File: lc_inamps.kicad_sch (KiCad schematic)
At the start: 30 parts, among them J14 Conn_01x04_Male, J15 Conn_01x04_Male, J16 Conn_01x04, J17 Conn_01x08, J18 Conn_01x04_Male, J19 Conn_01x04_Male, U3 MCP6N11R, U4 MCP6N11R, U5 MCP6N11R, U6 MCP6N11R

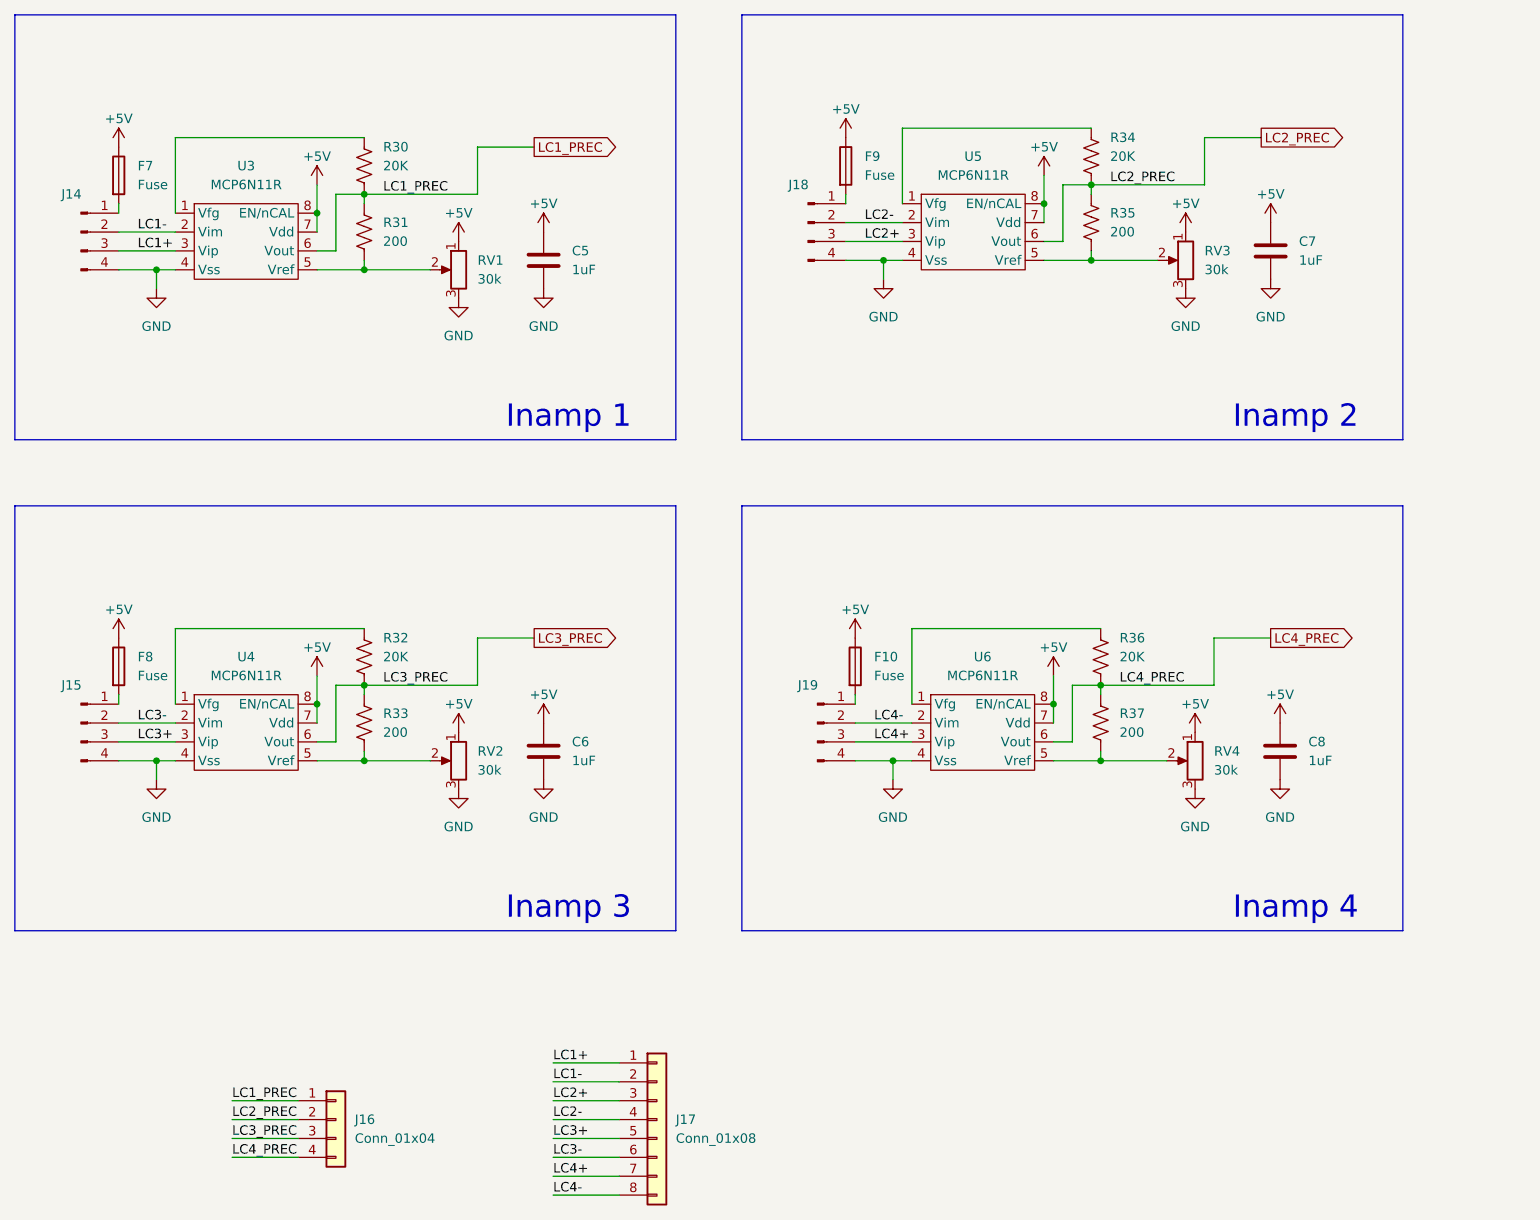
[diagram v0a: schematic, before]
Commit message: added footprints and started schematic review revisions
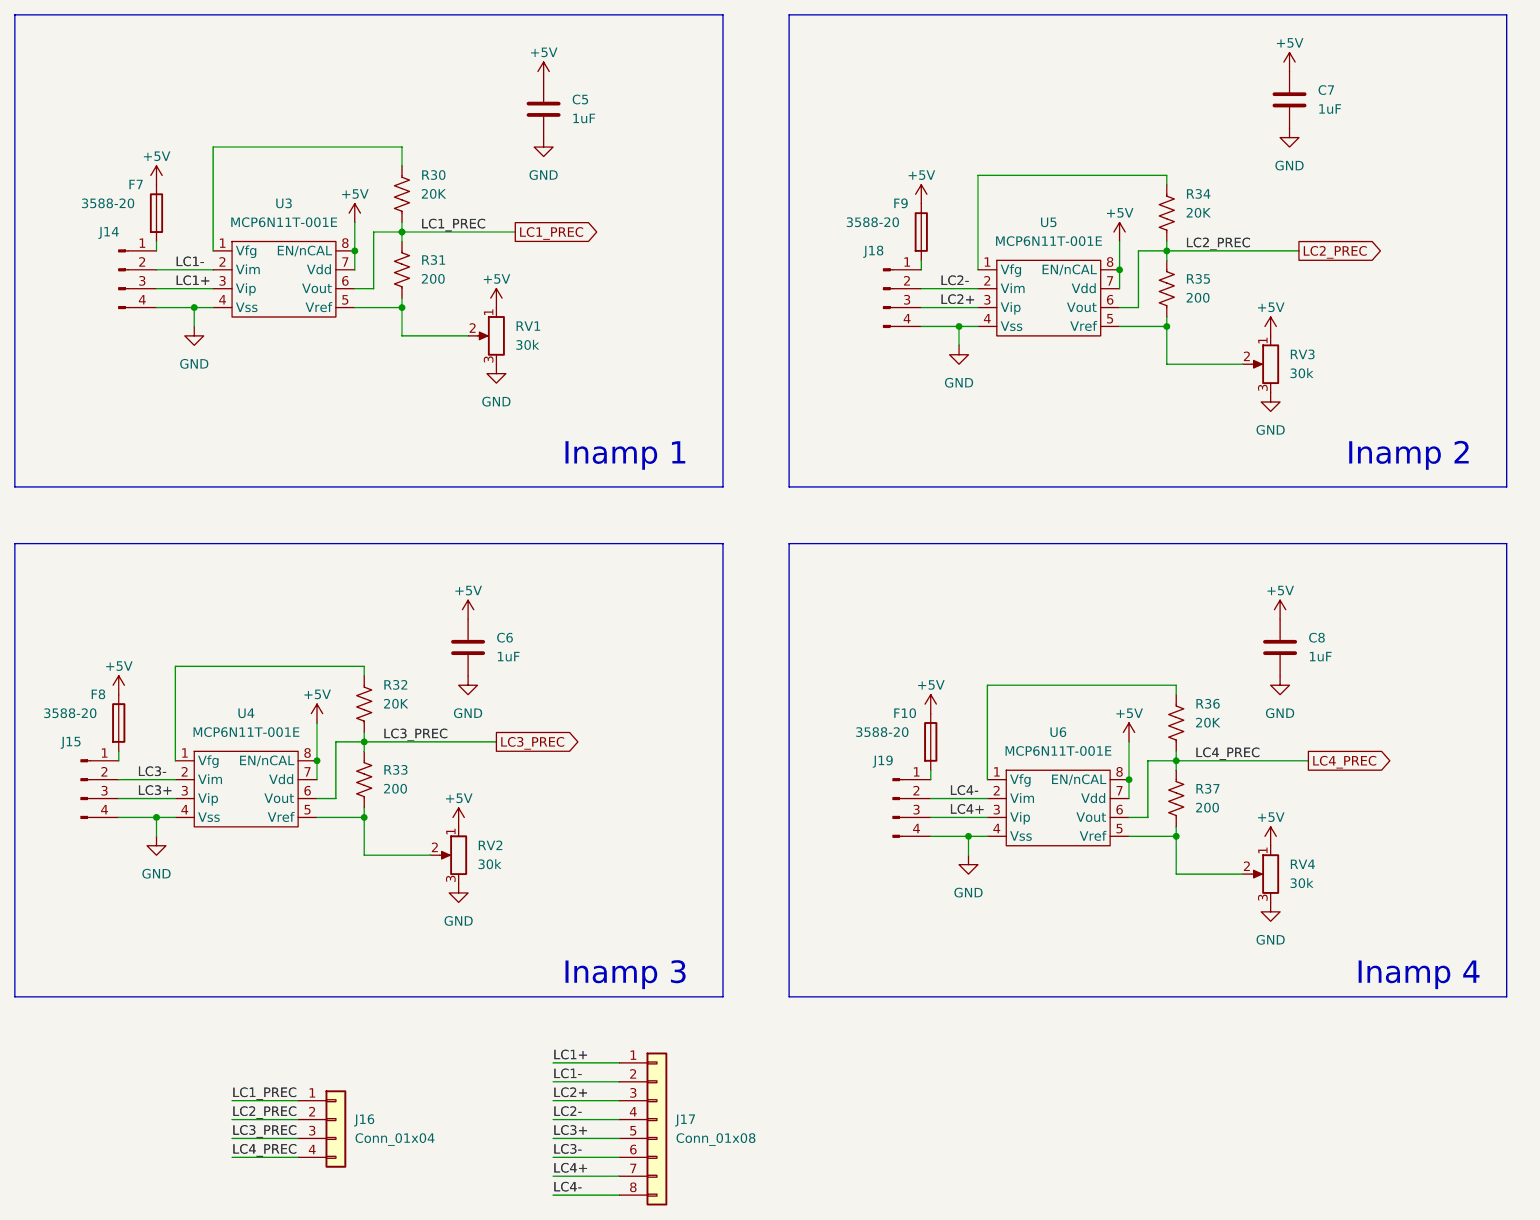
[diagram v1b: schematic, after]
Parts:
- C5, C6, C7, C8: footprint (none) -> Capacitor_SMD:C_1206_3216Metric
- F10, F7, F8, F9: value Fuse -> 3588-20; footprint (none) -> karca_custom_footprints:3588-20 fuse
- R30, R31, R32, R33, R34, R35, R36, R37, RV1, RV2, RV3, RV4: footprint (none) -> Resistor_SMD:R_1206_3216Metric
- U3, U4, U5, U6: value MCP6N11R -> MCP6N11T-001E; footprint (none) -> Package_DFN_QFN:TDFN-8-1EP_3x2mm_P0.5mm_EP1.80x1.65mm
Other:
- moved on the sheet: C5, C6, C7, C8, F10, F7, F8, F9, J14, J15, J18, J19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
